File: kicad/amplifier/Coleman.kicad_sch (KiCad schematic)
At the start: 0 parts

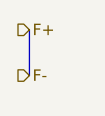
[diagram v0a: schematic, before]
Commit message: kicad work
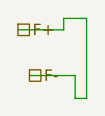
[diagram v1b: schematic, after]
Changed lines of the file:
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@@
 (kicad_sch (version 20230121) (generator eeschema)
   (paper "A4")
-  (bus (pts (xy 148.59 73.66) (xy 148.59 78.74))
+  (wire (pts (xy 152.4 72.39) (xy 154.94 72.39))
     (stroke (width 0) (type default))
   )
-  (hierarchical_label "F+" (shape output) (at 147.32 73.66 0) (fields_autoplaced)
+  (wire (pts (xy 154.94 81.28) (xy 153.67 81.28))
+    (stroke (width 0) (type default))
+  )
+  (wire (pts (xy 148.59 78.74) (xy 153.67 78.74))
+    (stroke (width 0) (type default))
+  )
+  (wire (pts (xy 152.4 73.66) (xy 152.4 72.39))
+    (stroke (width 0) (type default))
+  )
+  (wire (pts (xy 147.32 73.66) (xy 152.4 73.66))
+    (stroke (width 0) (type default))
+  )
+  (wire (pts (xy 153.67 81.28) (xy 153.67 78.74))
+    (stroke (width 0) (type default))
+  )
+  (wire (pts (xy 154.94 72.39) (xy 154.94 81.28))
+    (stroke (width 0) (type default))
+  )
+  (hierarchical_label "F+" (shape passive) (at 147.32 73.66 0) (fields_autoplaced)
     (effects (font (size 1.27 1.27)) (justify left))
   )
-  (hierarchical_label "F-" (shape output) (at 147.32 78.74 0) (fields_autoplaced)
+  (hierarchical_label "F-" (shape passive) (at 148.59 78.74 0) (fields_autoplaced)
     (effects (font (size 1.27 1.27)) (justify left))
   )
